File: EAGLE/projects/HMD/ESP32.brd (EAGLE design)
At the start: 43 x 38.5 mm, 40 parts, among them Q3 BSS138, Q4 BSS138, U3 LIS3DHTR, U4 MIC5225-3.3

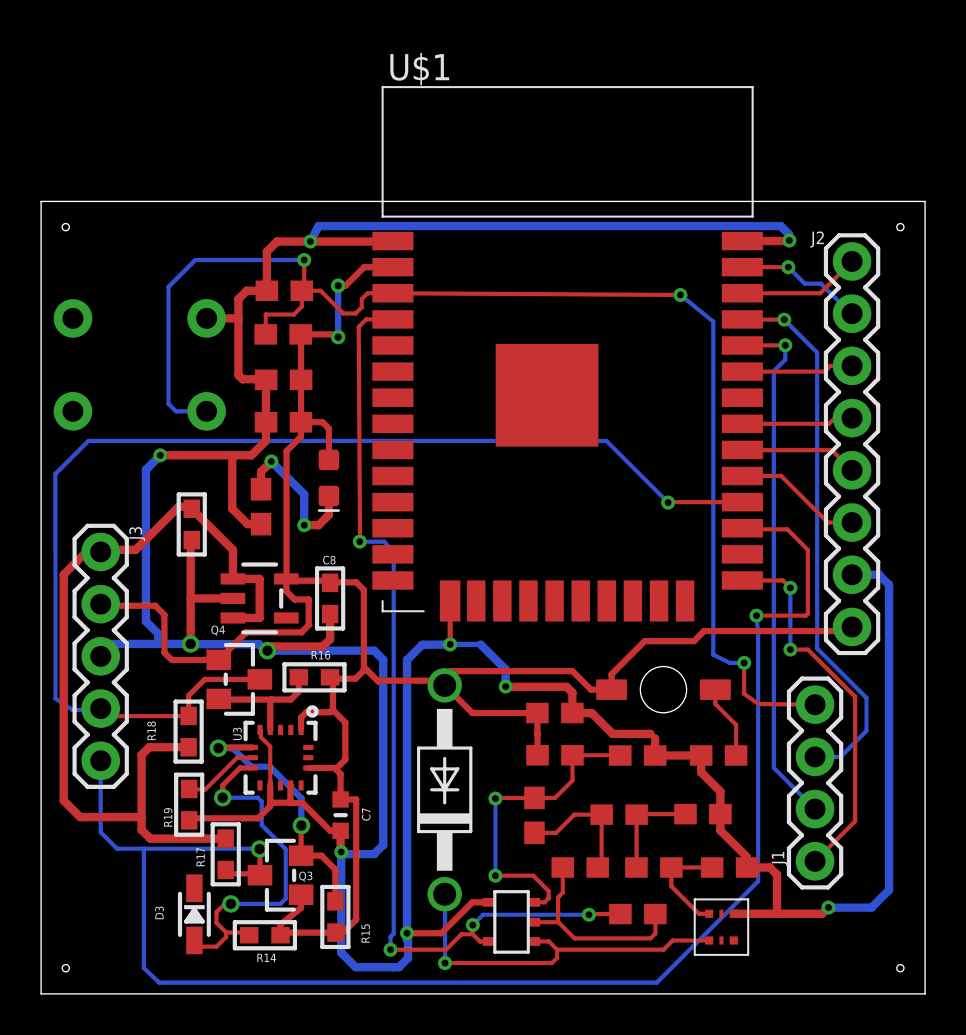
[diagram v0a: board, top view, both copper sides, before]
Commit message: Version 1 micro
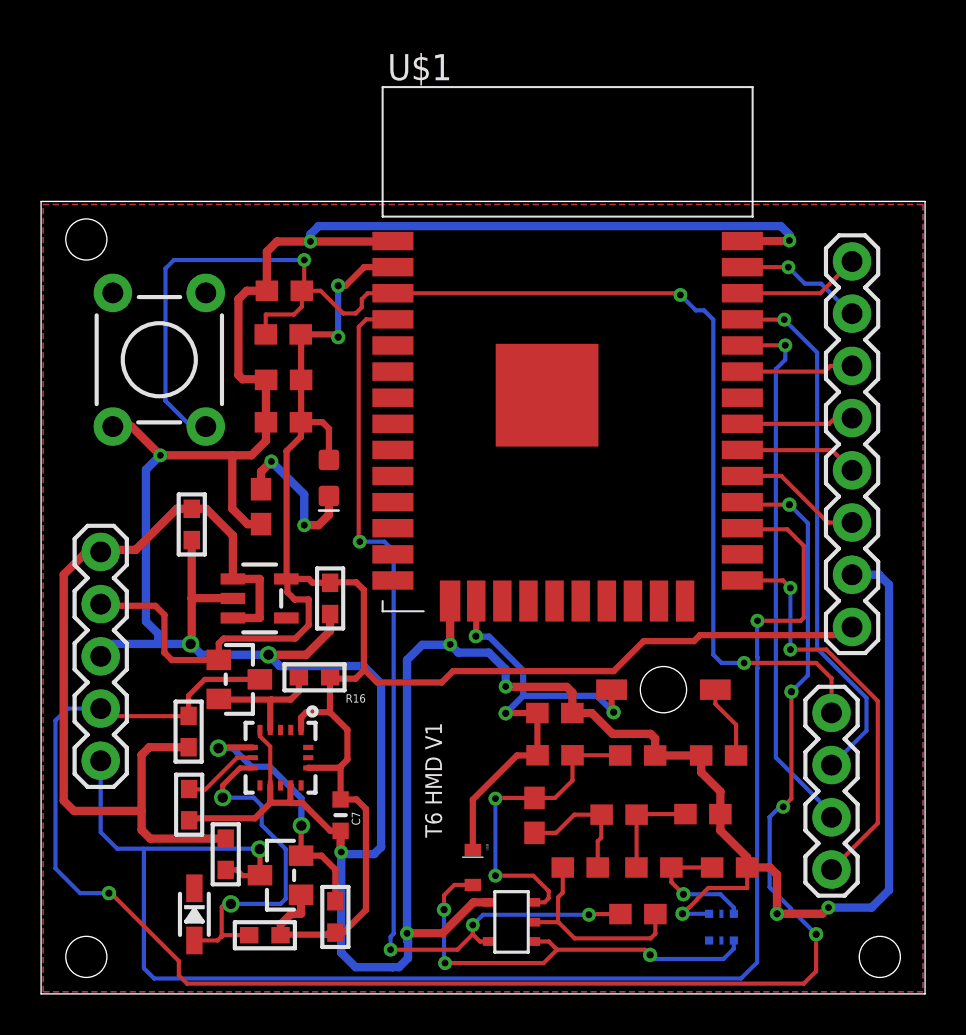
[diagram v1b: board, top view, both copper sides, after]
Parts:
- removed D2: 1N4004, diode:DO41-10
- added U$8: DI0603, HMD_Library:DIODE0603
- moved S1 0.98 mm to (5.75, 30.9), flipped to the top, turned to 90 degrees
- moved J1 0.89 mm to (38.5, 6.05)
- flipped U$6 to the bottom
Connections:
- new net HR_IN: C9.1, R11.1, U$1.P$16, U$7.P$1, U$8.P$1
- net 3.3V: no longer C9.1, D2.A, R11.1, U$7.P$1
- net N$16: now also U$8.P$2; no longer D2.C
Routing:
- net SCL: track 57.9 -> 86.2 mm, vias 1 -> 5
- net HR_IN: track 0.00 -> 23.1 mm, vias 0 -> 3
- net 3.3V: track 105.7 -> 97.9 mm
- net GND: track 199.9 -> 203.9 mm, vias 10 -> 12
- net N$16: track 18.2 -> 21.4 mm, vias 1 -> 3
- net EN: track 64.6 -> 67.0 mm
- net SDA: track 74.8 -> 76.6 mm
- net N$7: track 18.4 -> 19.9 mm
- net N$9: track 5.29 -> 6.55 mm, vias 0 -> 1
- net N$1: track 17.7 -> 17.0 mm
- net PTX: track 25.7 -> 26.4 mm
- net PRX: track 26.7 -> 26.1 mm
- added copper zone on layer 1, net GND
- added copper zone on layer 16, net GND
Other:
- board text added: "T6 HMD V1"
- board text removed: "LIS3DH"

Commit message: Revert "Version 1 micro"
This reverts commit 22c8d65d876e5e97d8f3c243cdc0f8aa191d734f.
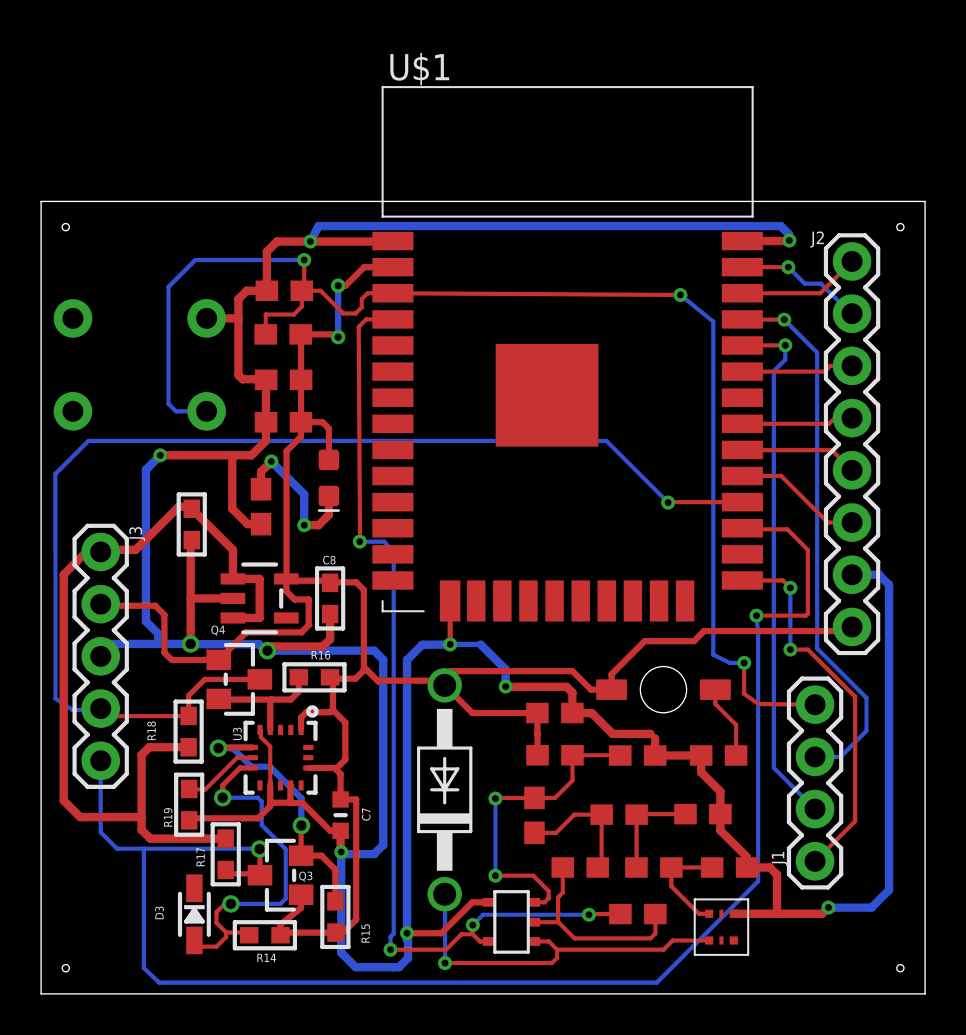
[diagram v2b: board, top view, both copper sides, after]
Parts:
- removed U$8: DI0603, HMD_Library:DIODE0603
- added D2: 1N4004, diode:DO41-10
- moved S1 0.98 mm to (4.80, 30.6), flipped to the bottom, turned to 0 degrees
- moved J1 0.89 mm to (37.6, 6.45)
- flipped U$6 to the top
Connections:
- removed net HR_IN: C9.1, R11.1, U$1.P$16, U$7.P$1, U$8.P$1
- net 3.3V: now also C9.1, D2.A, R11.1, U$7.P$1
- net N$16: now also D2.C; no longer U$8.P$2
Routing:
- net SCL: track 86.2 -> 57.9 mm, vias 5 -> 1
- net HR_IN: track 23.1 -> 0.00 mm, vias 3 -> 0
- net 3.3V: track 97.9 -> 105.7 mm
- net GND: track 203.9 -> 199.9 mm, vias 12 -> 10
- net N$16: track 21.4 -> 18.2 mm, vias 3 -> 1
- net EN: track 67.0 -> 64.6 mm
- net SDA: track 76.6 -> 74.8 mm
- net N$7: track 19.9 -> 18.4 mm
- net N$9: track 6.55 -> 5.29 mm, vias 1 -> 0
- net N$1: track 17.0 -> 17.7 mm
- net PTX: track 26.4 -> 25.7 mm
- net PRX: track 26.1 -> 26.7 mm
- removed copper zone on layer 1, net GND
- removed copper zone on layer 16, net GND
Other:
- board text added: "LIS3DH"
- board text removed: "T6 HMD V1"
